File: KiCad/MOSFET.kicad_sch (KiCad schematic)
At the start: 6 parts, among them J7 Screw_Terminal_01x04, Q1 IRLZ44N

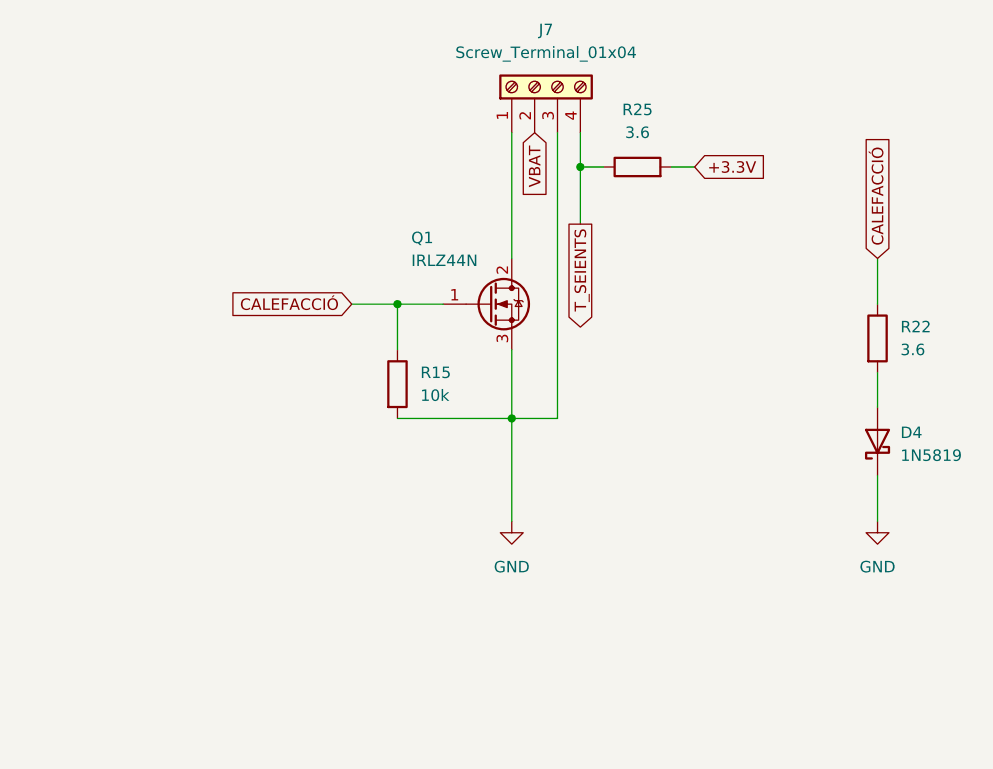
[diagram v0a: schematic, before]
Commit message: cambios en el mosfet
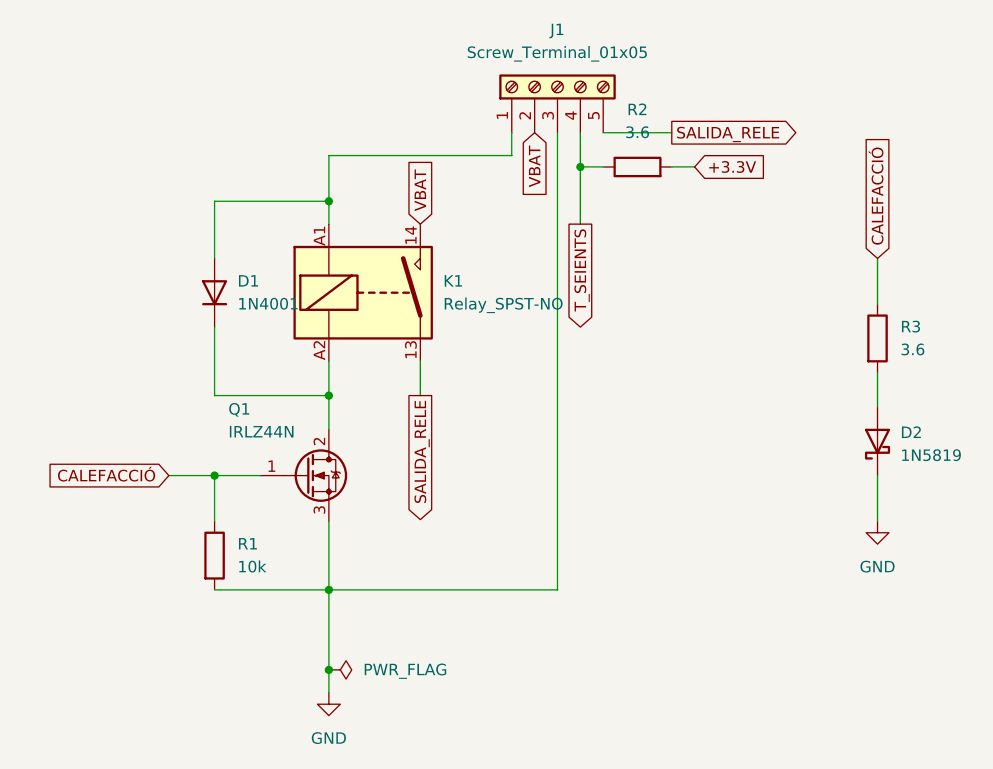
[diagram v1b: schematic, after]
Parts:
- removed J7: Screw_Terminal_01x04, TerminalBlock_Phoenix:TerminalBlock_Phoenix_MKDS-1,5-4-5.08_1x04_P5.08mm_Horizontal, symbol Connector:Screw_Terminal_01x04
- added D1: 1N4001, Diode_THT:D_DO-41_SOD81_P10.16mm_Horizontal, symbol Diode:1N4001
- added J1: Screw_Terminal_01x05, symbol Connector:Screw_Terminal_01x05
- added K1: Relay_SPST-NO, symbol Relay:Relay_SPST-NO
- renumbered D4 to D2, R15 to R1, R25 to R2, R22 to R3
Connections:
- net GND: now also J1.3 (Pin_3)
- net T_SEIENTS: now also J1.4 (Pin_4)
- net VBAT: now also J1.2 (Pin_2), K1.14
- net at Q1.2 (D): now also D1.1 (K), K1.A2
- new net: D1.2 (A), J1.1 (Pin_1), K1.A1
- new net SALIDA_RELE: J1.5 (Pin_5), K1.13
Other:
- moved on the sheet: Q1, R1
